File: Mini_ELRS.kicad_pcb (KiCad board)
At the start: 4 copper layers, 27.9 x 26.9 mm, 24 parts, among them J1 Conn_01x06, J2 Conn_01x06, J3 Conn_01x06, SW1 SW_Push, U1 ESP32-PICO-D4, U2 TC2014-3.3VxCTTR, U3 SX1280IMLTRT, Y1 Crystal_GND24_Small

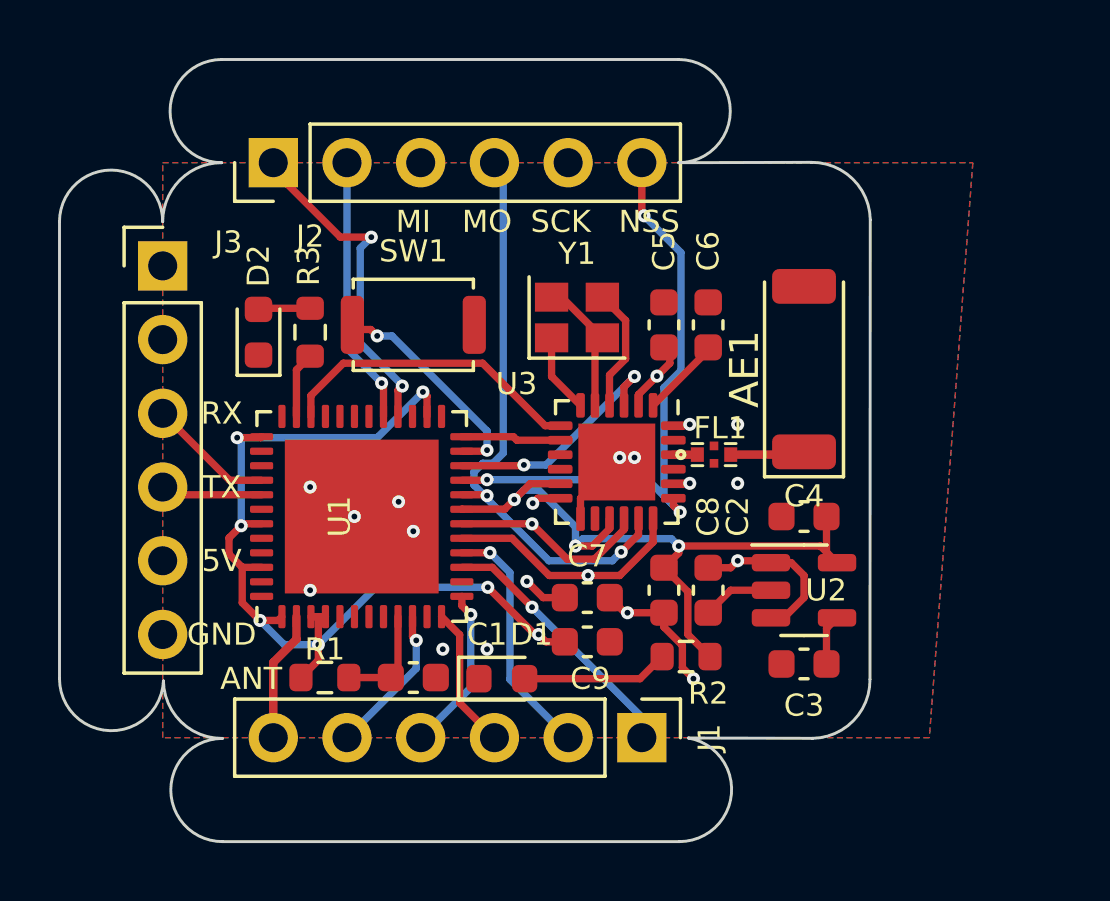
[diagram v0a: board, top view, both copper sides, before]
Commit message: update esp32_with_mos
Signed-off-by: huangzzk <huangcmzzk@gmail.com>
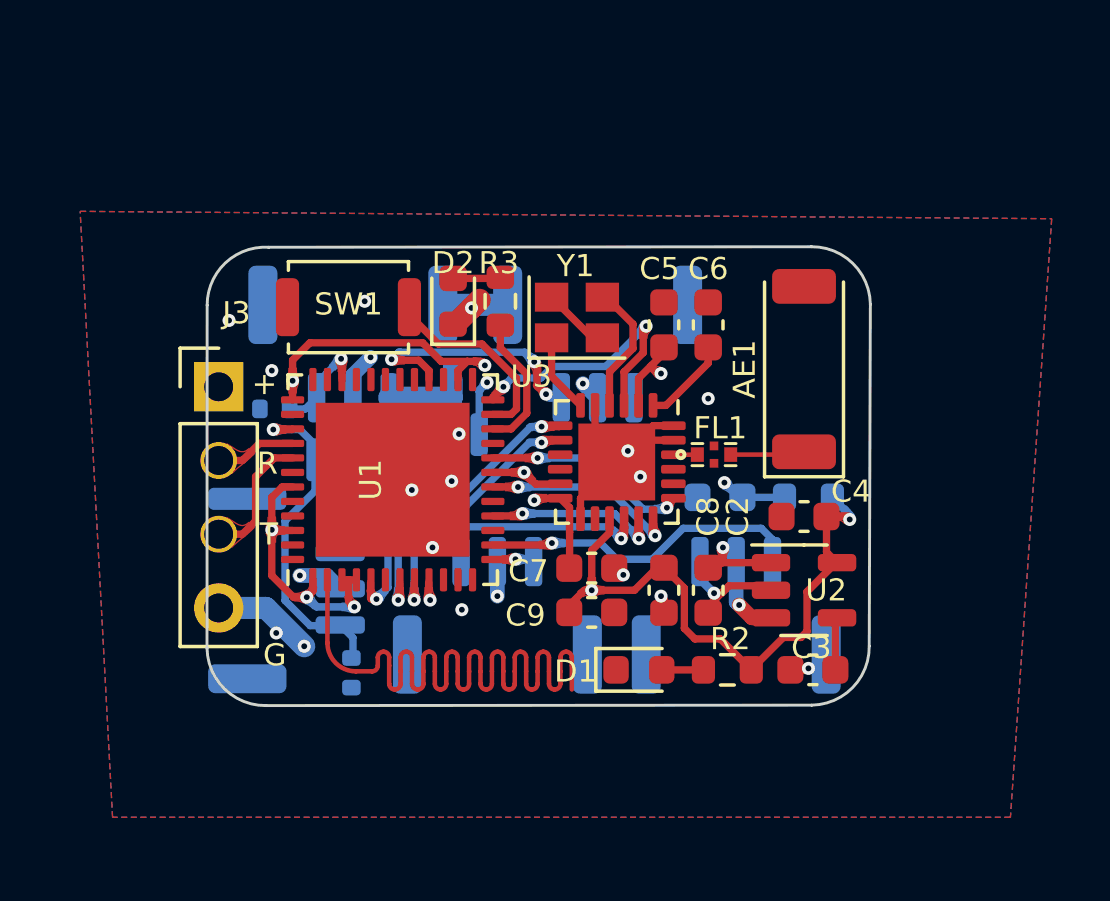
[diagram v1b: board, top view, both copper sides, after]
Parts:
- added J4: Conn_01x03_MountingPin, Connector_Molex:Molex_CLIK-Mate_502386-0370_1x03-1MP_P1.25mm_Horizontal, B.Cu at (119.8, 68.4)
- added J5: Conn_01x03, Connector_Molex:Molex_CLIK-Mate_502386-0370_1x03-1MP_P1.25mm_Horizontal, B.Cu at (111.6, 68.4)
- added J6: Conn_01x03_MountingPin, Connector_Molex:Molex_CLIK-Mate_502386-0370_1x03-1MP_P1.25mm_Horizontal, B.Cu at (115.1, 59.1)
- added Q1: Q_NMOS_GSD, Package_TO_SOT_SMD:SOT-23, B.Cu at (106.3, 64.0)
- added Q2: Q_NMOS_GSD, Package_TO_SOT_SMD:SOT-23, B.Cu at (110.0, 61.3)
- added R4: 10K, Resistor_SMD:R_0402_1005Metric, B.Cu at (106.6, 70.4)
- added R5: 10K, Resistor_SMD:R_0402_1005Metric, B.Cu at (103.9, 61.3)
- C1, R1: moved to B.Cu
- J1, J2: value Conn_01x06 -> Conn_01x03_MountingPin; footprint Connector_PinHeader_2.54mm:PinHeader_1x06_P2.54mm_Vertical -> Connector_Molex:Molex_CLIK-Mate_502386-0370_1x03-1MP_P1.25mm_Horizontal; moved to B.Cu
- J3: value Conn_01x06 -> Conn_01x04; footprint Connector_PinHeader_2.54mm:PinHeader_1x06_P2.54mm_Vertical -> Connector_PinHeader_2.54mm:PinHeader_1x04_P2.54mm_Vertical
- moved R1 17.8 mm to (122.3, 64.4), turned to 180 degrees
- moved J1 13.3 mm to (104.3, 67.5), turned to 90 degrees
- moved C1 12.3 mm to (119.3, 64.4), turned to 180 degrees
- moved J2 6.82 mm to (106.6, 59.1), turned to 0 degrees
- moved D2 6.79 mm to (110.1, 57.6)
- moved R3 6.64 mm to (111.7, 57.6)
- moved D1 4.73 mm to (116.5, 70.3)
- moved J3 4.59 mm to (102.0, 60.6)
- moved SW1 2.32 mm to (106.5, 57.8), turned to 180 degrees
- moved U1 1.66 mm to (108.0, 63.8)
- moved R2 1.49 mm to (119.5, 70.3)
- moved C9 1.03 mm to (114.9, 68.3)
- moved C7 1.03 mm to (114.9, 66.8)
- moved C3 0.37 mm to (122.5, 70.3)
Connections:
- C2 pad 1: +5V -> +BATT
- J1 pad 1: Net-(J1-Pad1) -> /PWM1
- J1 pad 2: Net-(J1-Pad2) -> +BATT
- J1 pad 3: Net-(J1-Pad3) -> Net-(Q1-Pad3)
- J2 pad 1: Net-(J2-Pad1) -> /PWM2
- J2 pad 2: Net-(J2-Pad2) -> +BATT
- J2 pad 3: /MISO -> Net-(Q2-Pad3)
- J3 pad 1: unconnected-(J3-Pad1) -> +BATT
- J3 pad 2: unconnected-(J3-Pad2) -> /RX
- J3 pad 3: /RX -> /TX
- J3 pad 4: /TX -> GND
- U1 pad 10: Net-(J1-Pad5) -> unconnected-(U1-Pad10)
- U1 pad 12: Net-(J1-Pad3) -> /PWM7
- U1 pad 13: Net-(J1-Pad4) -> /PWM4
- U1 pad 14: unconnected-(U1-Pad14) -> /PWM3
- U1 pad 15: Net-(J1-Pad1) -> unconnected-(U1-Pad15)
- U1 pad 16: Net-(J1-Pad2) -> /MOSI
- U1 pad 17: /SCK -> unconnected-(U1-Pad17)
- U1 pad 18: /MISO -> /SCK
- U1 pad 20: /MOSI -> /NSS
- U1 pad 21: /NSS -> unconnected-(U1-Pad21)
- U1 pad 22: /NRST -> /LED
- U1 pad 24: /DIO1 -> /NRST
- U1 pad 28: Net-(J2-Pad1) -> /PWM5
- U1 pad 29: Net-(J2-Pad2) -> unconnected-(U1-Pad29)
- U1 pad 34: /BUSY -> /PWM2
- U1 pad 35: /LED -> unconnected-(U1-Pad35)
- U1 pad 36: unconnected-(U1-Pad36) -> /PWM6
- U1 pad 39: unconnected-(U1-Pad39) -> /PWM1
- U1 pad 42: unconnected-(U1-Pad42) -> /PWM8
- U1 pad 5: unconnected-(U1-Pad5) -> /BUSY
- U1 pad 7: unconnected-(U1-Pad7) -> /DIO1
- U1 pad 8: unconnected-(U1-Pad8) -> /MISO
- U2 pad 1: +5V -> +BATT
- U2 pad 3: +5V -> +BATT
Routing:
- net +5V: track 28.5 -> 0.00 mm, vias 1 -> 0
- net /ESP32_ANT: track 4.50 -> 30.7 mm
- net /SCK: track 27.3 -> 6.91 mm, vias 1 -> 2
- net /NSS: track 21.6 -> 7.17 mm, vias 3 -> 2
- net /MOSI: track 20.5 -> 6.14 mm
- net +BATT: track 0.00 -> 13.1 mm, vias 0 -> 8
- net Net-(C1-Pad1): track 3.65 -> 15.6 mm, vias 0 -> 2
- net /PWM1: track 0.00 -> 11.8 mm, vias 0 -> 1
- net Net-(J2-Pad1): track 11.6 -> 0.00 mm, vias 2 -> 0
- net /PWM3: track 0.00 -> 11.3 mm, vias 0 -> 1
- net /MISO: track 21.6 -> 10.8 mm, vias 1 -> 2
- net /PWM2: track 0.00 -> 10.8 mm, vias 0 -> 2
- net GND: track 14.5 -> 24.6 mm, vias 15 -> 16
- net Net-(J2-Pad2): track 9.26 -> 0.00 mm, vias 1 -> 0
- net Net-(J1-Pad1): track 9.05 -> 0.00 mm, vias 1 -> 0
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- added copper zone on In2.Cu, net +BATT
- removed copper zone on In2.Cu, net GND
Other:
- board size 27.9 x 26.9 mm -> 22.9 x 15.8 mm
- board text added: "+"
- board text added: "G"
- board text added: "PWM1"
- board text added: "PWM2"
- board text added: "PWM3"
- board text added: "PWM4"
- board text added: "PWM5"
- board text added: "R"
- board text added: "T"
- board text removed: "5V"
- board text removed: "ANT"
- board text removed: "GND"
- board text removed: "MI"
- board text removed: "MO"
- board text removed: "NSS"
- board text removed: "RX"
- board text removed: "SCK"
- board text removed: "TX"
